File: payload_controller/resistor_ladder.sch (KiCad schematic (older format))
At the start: 34 parts, among them U1 74HC590, U10 ADG841YKSZ-500RL7, U11 ADG841YKSZ-500RL7, U11 MCP4725xxx-xCH, U12 ADG841YKSZ-500RL7, U13 ADG841YKSZ-500RL7, U6 ADG841YKSZ-500RL7, U7 ADG841YKSZ-500RL7, U8 ADG841YKSZ-500RL7, U9 ADG841YKSZ-500RL7

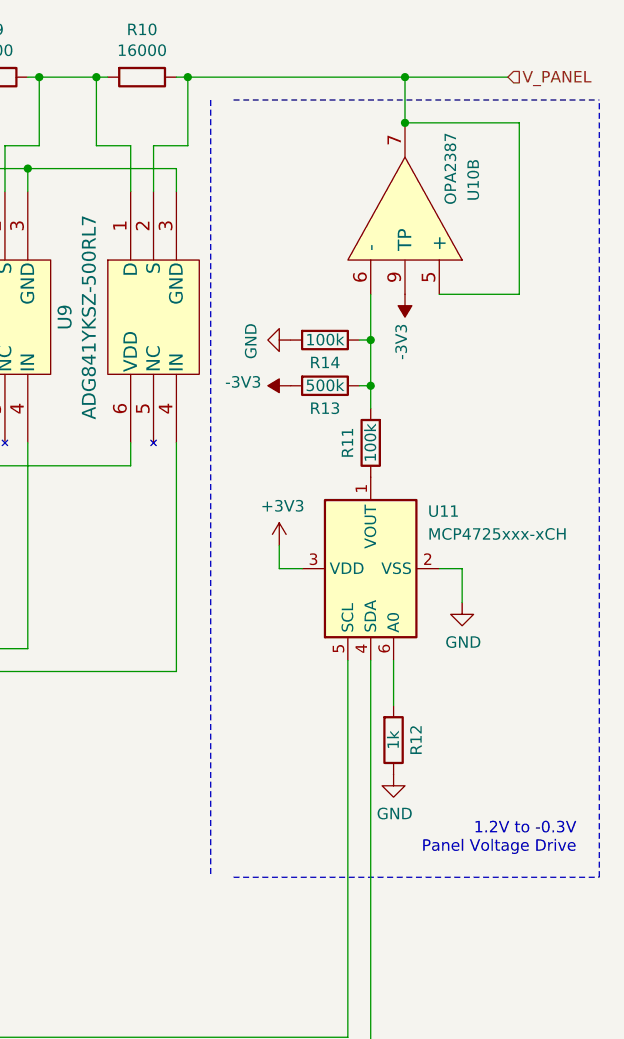
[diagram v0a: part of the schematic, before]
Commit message: Generated manufacturing files
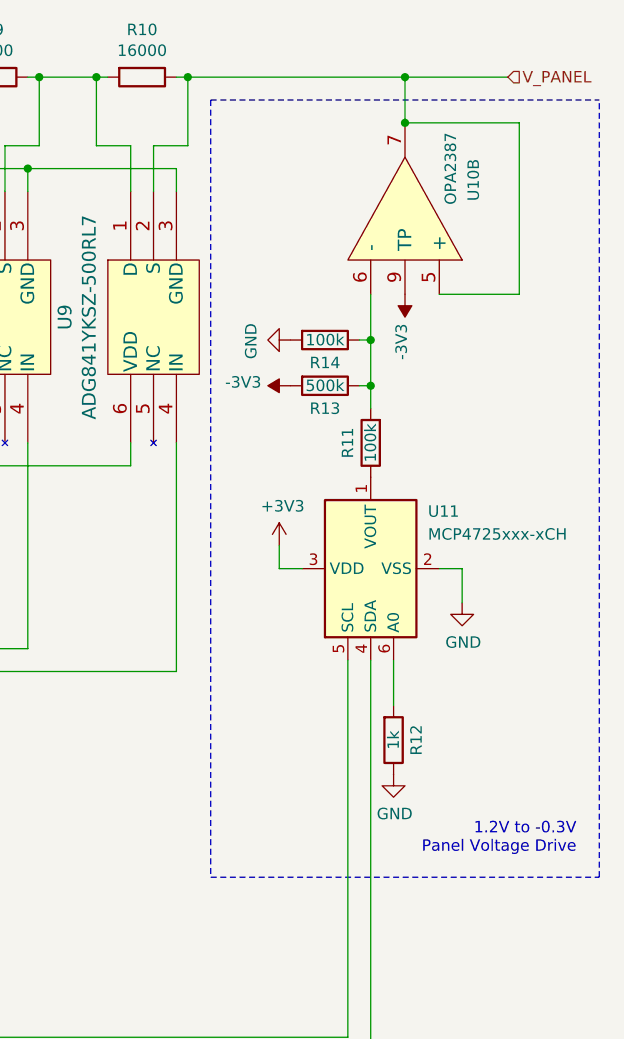
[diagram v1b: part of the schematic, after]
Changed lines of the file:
@@
 Sheet 2 6
 Title "Resistor 8-Bit Ladder"
-Date "2022-09-18"
+Date "2022-11-30"
 Rev "B"
 Comp "Advanced eXperimental Payloads | UNL Aerospace Club"
 Comment1 "Copyright (c) 2022"
 Comment2 "Designer: WSA"
-Comment3 "Reviewer:"
-Comment4 "Approved: "
+Comment3 "Reviewer: WSA"
+Comment4 "Approved: WSA"
 $EndDescr
 $Comp
@@
 	8650 1450 8650 4850
 Wire Notes Line
-	8750 4850 10350 4850
-Wire Notes Line
 	10350 4850 10350 1450
-Wire Notes Line
-	8750 1450 10350 1450
 Text Notes 10250 4750 2    50   ~ 0
 1.2V to -0.3V\nPanel Voltage Drive
@@
 	0    1    1    0
 $EndComp
+Wire Notes Line
+	8650 4850 10350 4850
+Wire Notes Line
+	8650 1450 10350 1450
 $EndSCHEMATC
